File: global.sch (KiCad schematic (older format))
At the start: 37 parts, among them Q5 MMBT3904, U11 74HC165, U12 74HC595, U13 74HC595, U14 74HC595, U5 74HCT125

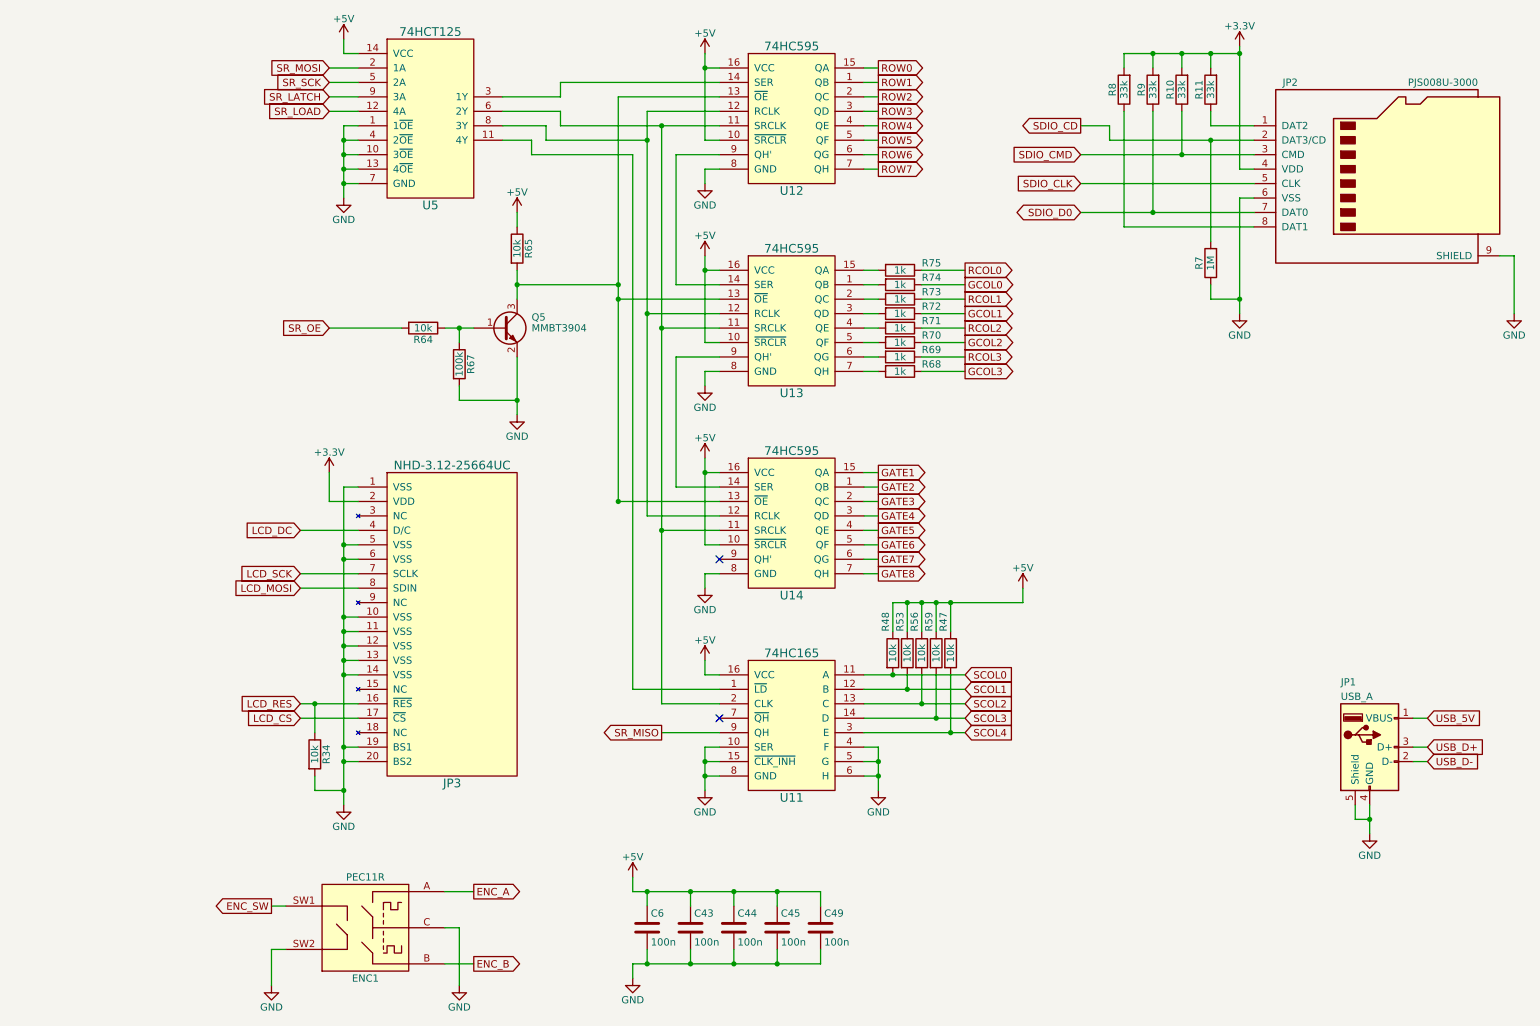
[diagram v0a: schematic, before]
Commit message: cleaned up schematics
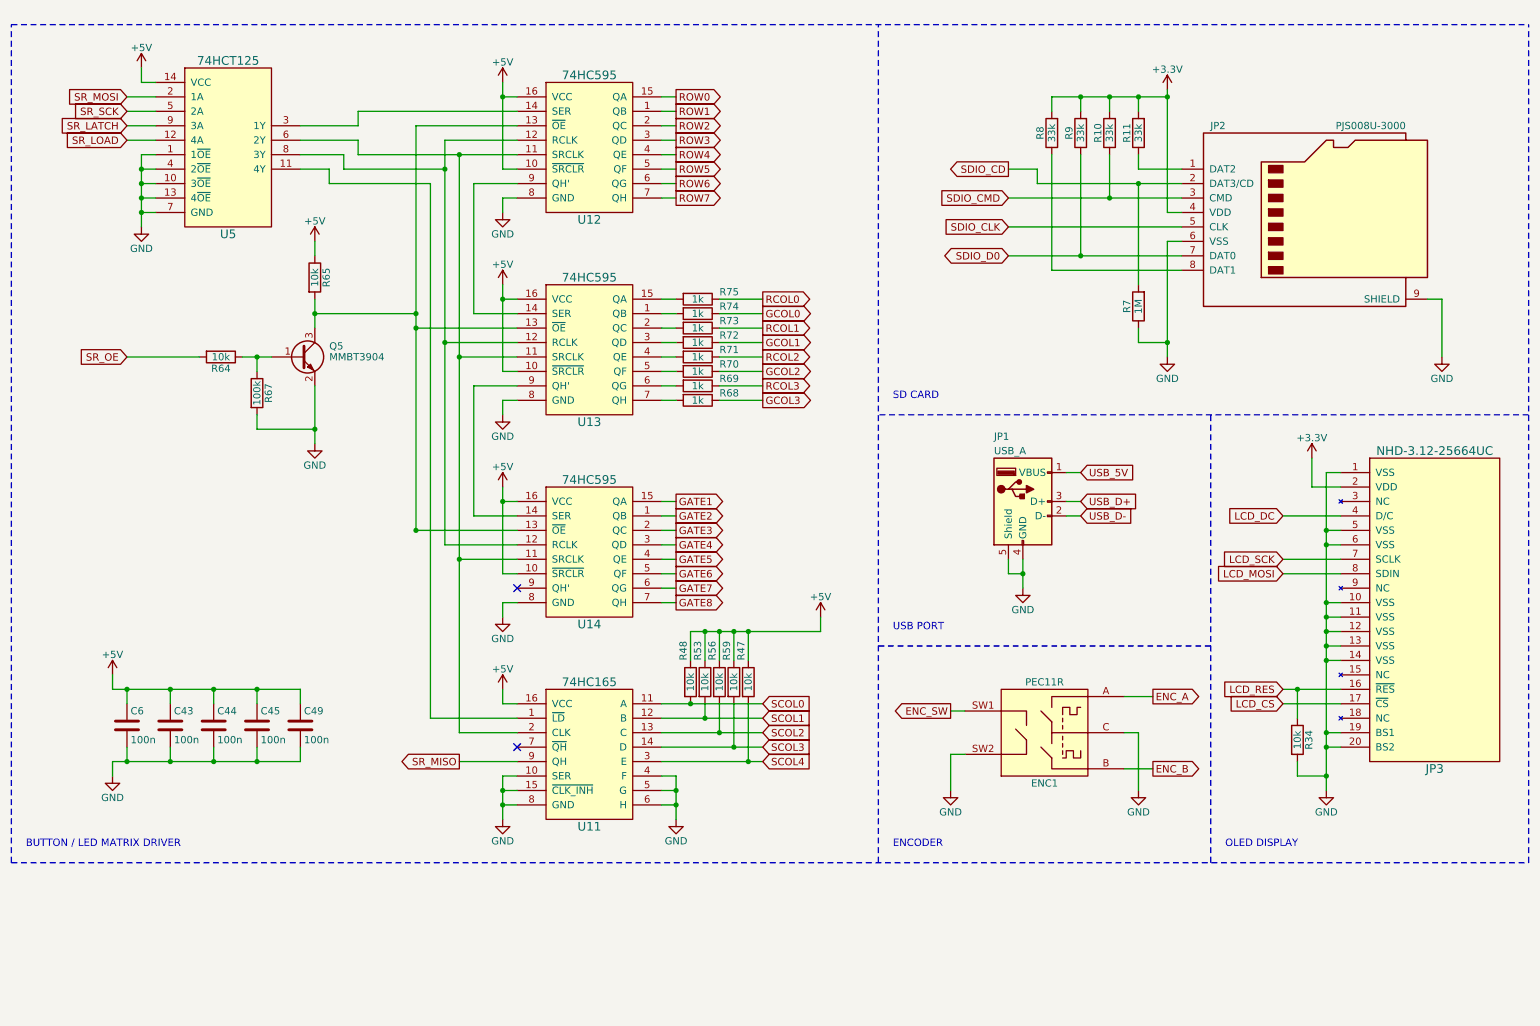
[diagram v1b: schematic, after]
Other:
- note added: "BUTTON / LED MATRIX DRIVER"
- note added: "ENCODER"
- note added: "OLED DISPLAY"
- note added: "SD CARD"
- note added: "USB PORT"
- moved on the sheet: C43, C44, C45, C49, C6, ENC1, JP1, JP2, JP3, Q5, R10, R11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
